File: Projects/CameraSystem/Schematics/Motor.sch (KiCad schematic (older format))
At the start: 3 parts, among them J13 Conn_02x02_Odd_Even, J14 Conn_02x05_Odd_Even

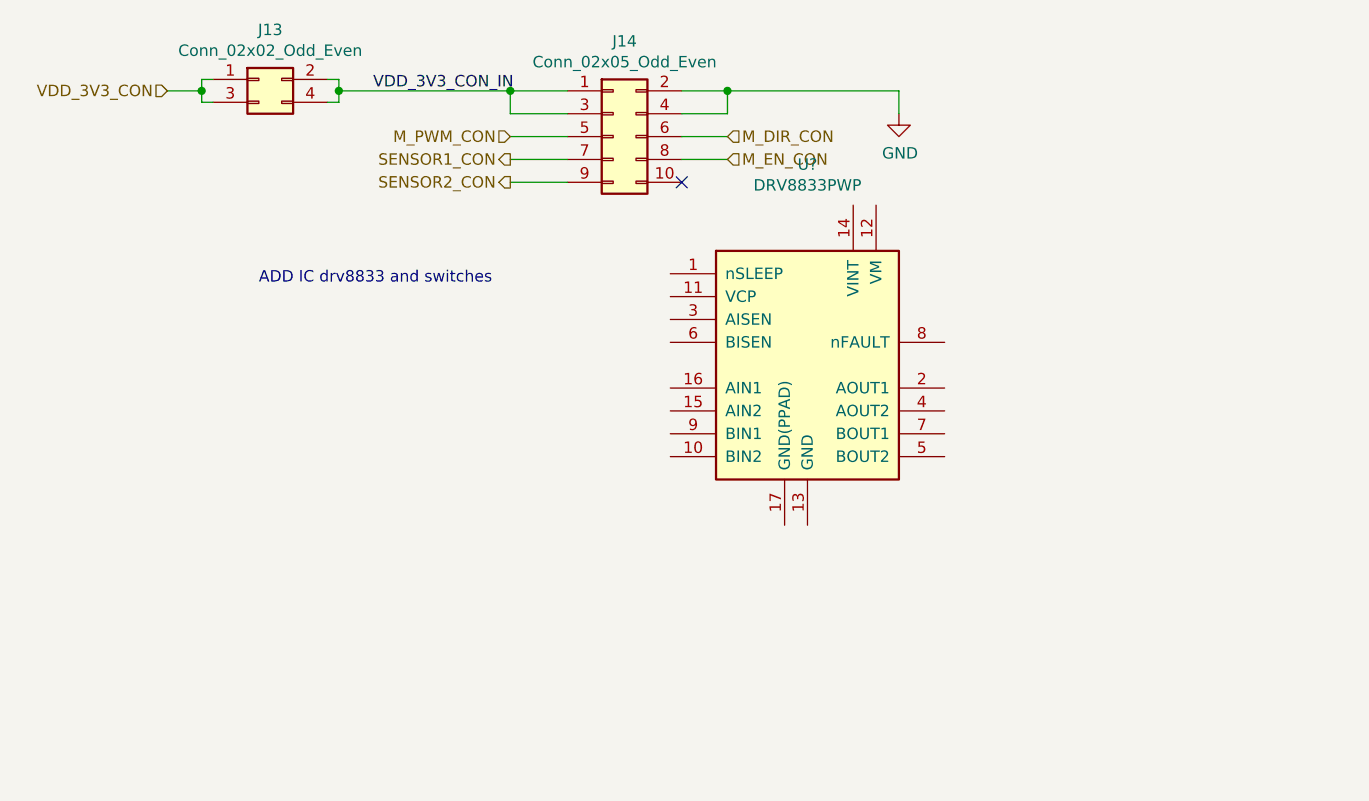
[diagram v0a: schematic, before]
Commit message: schematic updated
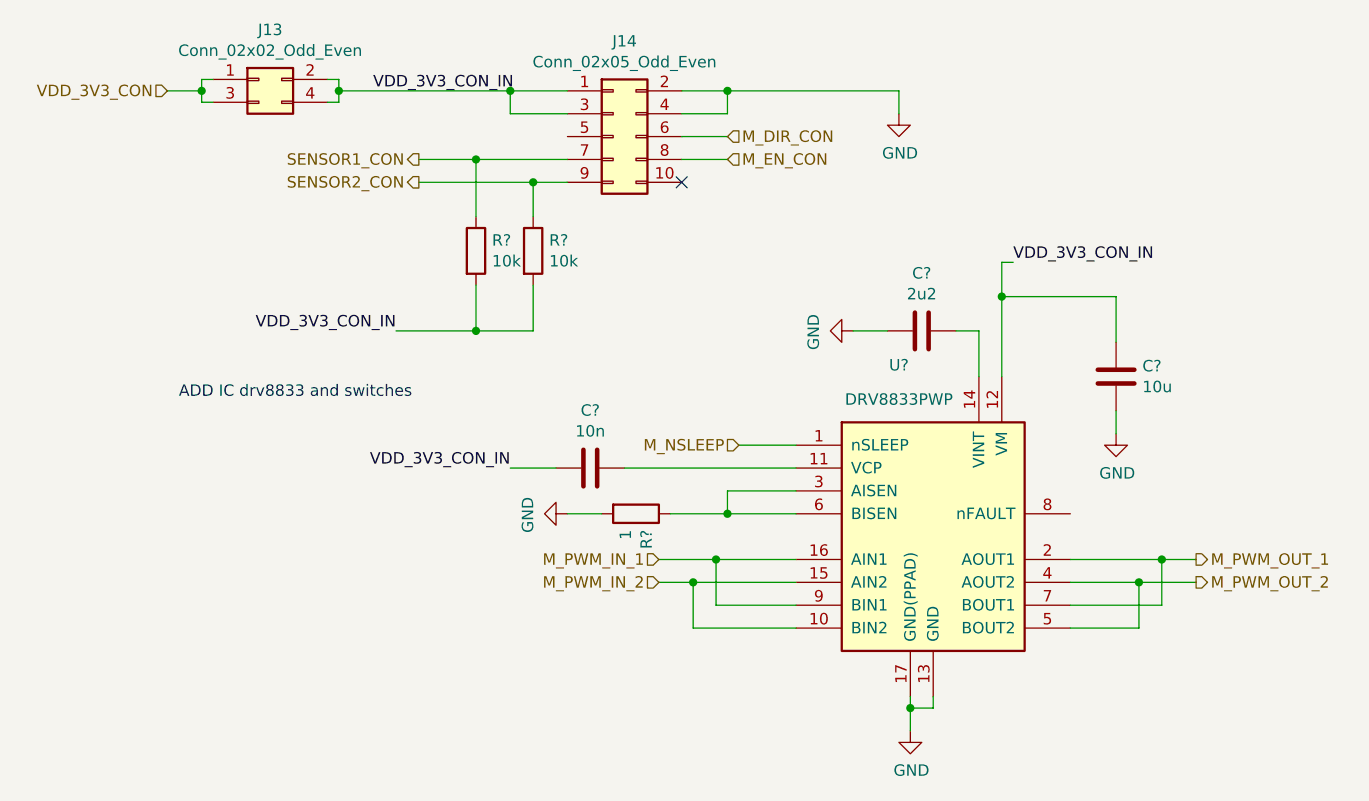
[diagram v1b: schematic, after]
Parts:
- added C?: 10u, symbol Device:C
- added C?: 10n, symbol Device:C
- added C?: 2u2, symbol Device:C
- added R? (x2): 10k, symbol Device:R
- added R?: 1, symbol Device:R
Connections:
- net GND: now also U?.13 (GND), U?.17 (GND(PPAD)), C?.1, C?.2, R?.2
- net SENSOR1_CON: now also R?.1
- net SENSOR2_CON: now also R?.1
- net VDD_3V3_CON_IN: now also U?.12 (VM), C?.1, C?.2, R?.2, R?.2
- net M_NSLEEP: now reaches U?.1 (nSLEEP)
- net M_PWM_IN_2: now reaches U?.10 (BIN2)
- net M_PWM_IN_2: now also U?.15 (AIN2)
- net at U?.11 (VCP): now also C?.1
- net at U?.14 (VINT): now also C?.2
- net M_PWM_IN_1: now reaches U?.16 (AIN1)
- net M_PWM_IN_1: now also U?.9 (BIN1)
- net M_PWM_OUT_1: now reaches U?.2 (AOUT1)
- net M_PWM_OUT_1: now also U?.7 (BOUT1)
- net at U?.3 (AISEN): now also U?.6 (BISEN), R?.1
- net M_PWM_OUT_2: now reaches U?.4 (AOUT2)
- net M_PWM_OUT_2: now also U?.5 (BOUT2)
- net M_PWM_CON: no longer names the net of J14.5 (Pin_5)
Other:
- moved on the sheet: U?
